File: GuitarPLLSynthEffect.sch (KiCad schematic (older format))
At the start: 36 parts

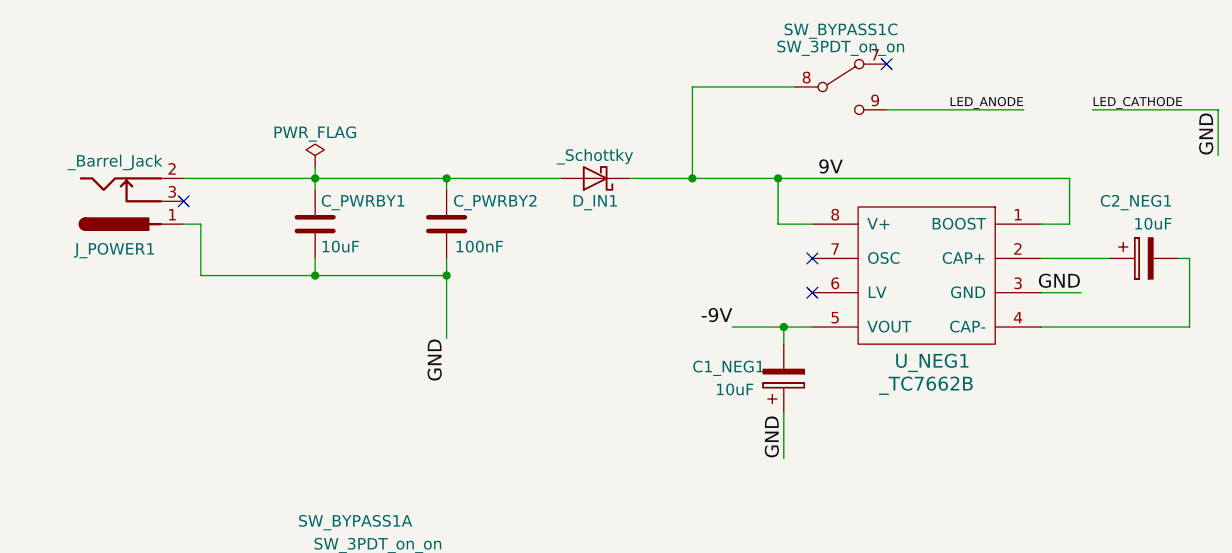
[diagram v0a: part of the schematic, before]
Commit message: Second draft PCB layout
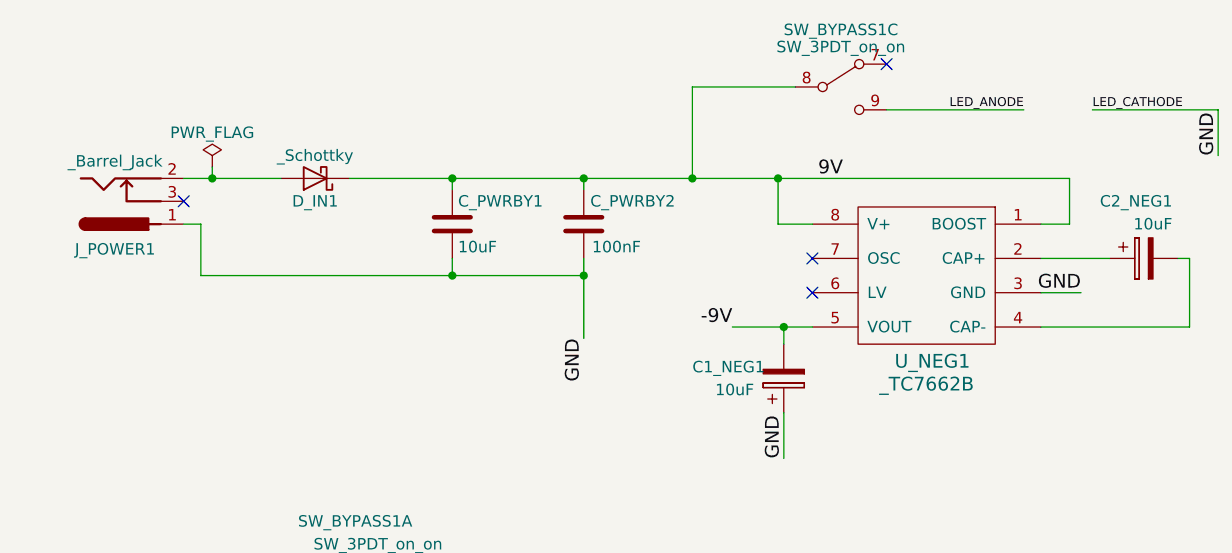
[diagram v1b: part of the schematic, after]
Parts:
- C_PWRBY1: footprint Capacitors_SMD:C_0805_HandSoldering -> Capacitors_SMD:CP_Elec_4x5.3
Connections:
- net 9V: now also C_PWRBY1.1, C_PWRBY2.2
- net at D_IN1.2 (A), J_POWER1.2: no longer C_PWRBY1.1, C_PWRBY2.2
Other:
- moved on the sheet: C_PWRBY1, C_PWRBY2, D_IN1
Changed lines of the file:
@@
 	1    0    0    1
 $EndComp
-Text Label 2625 2100 3    60   ~ 0
+Text Label 3225 2100 3    60   ~ 0
 GND
 Text Label 4250 1400 0    60   ~ 0
@@
 Wire Wire Line
 	9950 5500 9950 5975
-Wire Wire Line
-	2050 1350 2050 1450
-Connection ~ 2050 1400
+Connection ~ 2650 1400
 Wire Wire Line
 	4075 1400 4075 1600
@@
 Optional clean signal for FX
 Wire Wire Line
-	1475 1400 3125 1400
-Wire Wire Line
-	3425 1400 5350 1400
+	2200 1400 5350 1400
 $Comp
 L _Schottky D_IN1
 U 1 1 5AC34A74
-P 3275 1400
-F 0 "D_IN1" H 3275 1500 50  0000 C CNN
-F 1 "_Schottky" H 3275 1300 50  0000 C CNN
-F 2 "Diodes_SMD:D_SOD-123F" H 3275 1400 50  0001 C CNN
-F 3 "" H 3275 1400 50  0001 C CNN
-	1    3275 1400
+P 2050 1400
+F 0 "D_IN1" H 2050 1500 50  0000 C CNN
+F 1 "_Schottky" H 2050 1300 50  0000 C CNN
+F 2 "Diodes_SMD:D_SOD-123F" H 2050 1400 50  0001 C CNN
+F 3 "" H 2050 1400 50  0001 C CNN
+	1    2050 1400
 	-1   0    0    1
 $EndComp
@@
 	1550 1600 1550 1825
 Wire Wire Line
-	1550 1825 2625 1825
-Wire Wire Line
-	2625 1750 2625 2100
-Wire Wire Line
-	2050 1750 2050 1825
-Connection ~ 2050 1825
+	1550 1825 3225 1825
+Wire Wire Line
+	3225 1750 3225 2100
+Wire Wire Line
+	2650 1750 2650 1825
+Connection ~ 2650 1825
 $Comp
 L C C_PWRBY1
 U 1 1 5AC36CD5
-P 2050 1600
-F 0 "C_PWRBY1" H 2075 1700 50  0000 L CNN
-F 1 "10uF" H 2075 1500 50  0000 L CNN
-F 2 "Capacitors_SMD:C_0805_HandSoldering" H 2088 1450 50  0001 C CNN
-F 3 "" H 2050 1600 50  0001 C CNN
-	1    2050 1600
+P 2650 1600
+F 0 "C_PWRBY1" H 2675 1700 50  0000 L CNN
+F 1 "10uF" H 2675 1500 50  0000 L CNN
+F 2 "Capacitors_SMD:CP_Elec_4x5.3" H 2688 1450 50  0001 C CNN
+F 3 "" H 2650 1600 50  0001 C CNN
+	1    2650 1600
 	1    0    0    -1
 $EndComp
@@
 L PWR_FLAG #FLG01
 U 1 1 5AC38031
-P 2050 1350
-F 0 "#FLG01" H 2050 1425 50  0001 C CNN
-F 1 "PWR_FLAG" H 2050 1500 50  0000 C CNN
-F 2 "" H 2050 1350 50  0001 C CNN
-F 3 "" H 2050 1350 50  0001 C CNN
-	1    2050 1350
+P 1600 1350
+F 0 "#FLG01" H 1600 1425 50  0001 C CNN
+F 1 "PWR_FLAG" H 1600 1500 50  0000 C CNN
+F 2 "" H 1600 1350 50  0001 C CNN
+F 3 "" H 1600 1350 50  0001 C CNN
+	1    1600 1350
 	1    0    0    -1
 $EndComp
@@
 L C C_PWRBY2
 U 1 1 5AC5AF9D
-P 2625 1600
-F 0 "C_PWRBY2" H 2225 1500 50  0000 L CNN
-F 1 "100nF" H 2375 1700 50  0000 L CNN
-F 2 "Capacitors_SMD:C_0805_HandSoldering" H 2663 1450 50  0001 C CNN
-F 3 "" H 2625 1600 50  0001 C CNN
-	1    2625 1600
+P 3225 1600
+F 0 "C_PWRBY2" H 2825 1500 50  0000 L CNN
+F 1 "100nF" H 2975 1700 50  0000 L CNN
+F 2 "Capacitors_SMD:C_0805_HandSoldering" H 3263 1450 50  0001 C CNN
+F 3 "" H 3225 1600 50  0001 C CNN
+	1    3225 1600
 	-1   0    0    1
 $EndComp
 Wire Wire Line
-	2625 1450 2625 1400
-Connection ~ 2625 1400
-Connection ~ 2625 1825
+	3225 1450 3225 1400
+Connection ~ 3225 1400
+Connection ~ 3225 1825
+Wire Wire Line
+	1475 1400 1900 1400
+Wire Wire Line
+	1600 1350 1600 1400
+Connection ~ 1600 1400
+Wire Wire Line
+	2650 1450 2650 1400
 $EndSCHEMATC
